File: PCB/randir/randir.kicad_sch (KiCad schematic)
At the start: 15 parts, among them J1 JST connector, SW1 SW_Push, SW10 SW_Push, SW2 SW_Push, SW3 SW_Push, SW4 SW_Push, SW5 SW_Push, SW6 SW_Push, SW7 SW_Push, SW8 SW_Push, SW9 SW_Push, U1 nice_nano

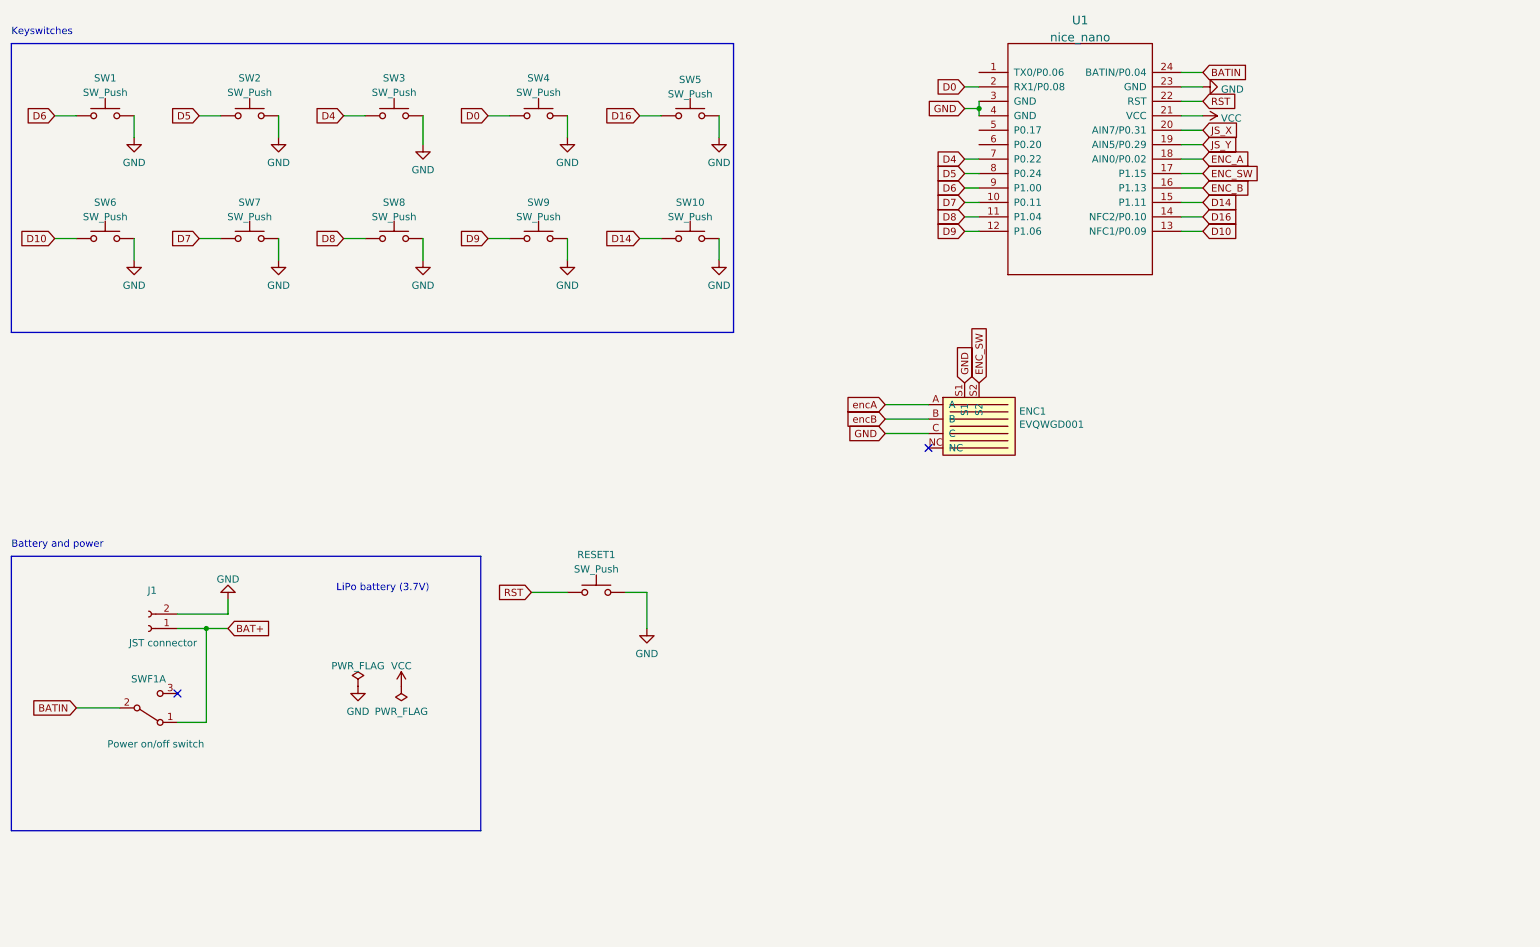
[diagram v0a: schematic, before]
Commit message: sides
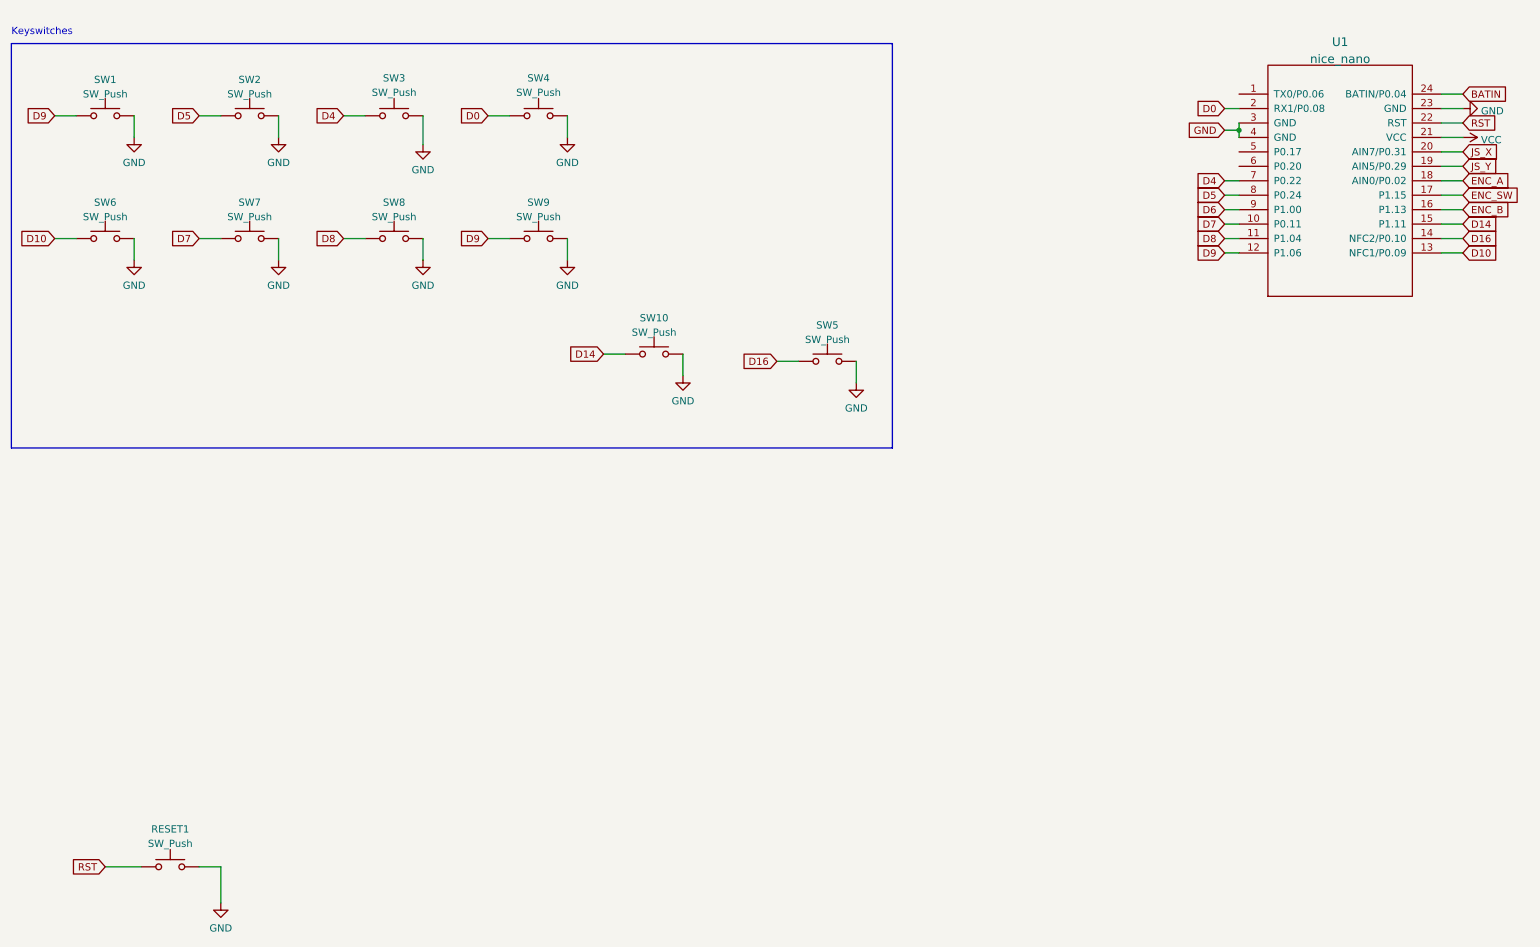
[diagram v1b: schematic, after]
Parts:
- removed ENC1: EVQWGD001, footprints:EVQWGD001, symbol chocofly-rescue:EVQWGD001-evqwgd001
- removed J1: JST connector, footprints:JST-ZH-2p-1.5, symbol Connector:Conn_01x02_Female
- removed SWF1: Power on/off switch, footprints:pwr-sw-smd-pcm12, symbol Switch:SW_DPDT_x2
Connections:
- net D6: no longer SW1.1
- net D9: now also SW1.1
- no-connect marks 2 -> 0
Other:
- note removed: "Battery and power"
- note removed: "LiPo battery (3.7V)"
- moved on the sheet: RESET1, SW10, SW5, U1
